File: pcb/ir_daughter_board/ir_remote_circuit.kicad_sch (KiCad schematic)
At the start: 12 parts, among them J2 Conn_01x06, J3 Conn_01x06, SW1 BOOT, SW2 RESET, U3 ESP-WROOM-02

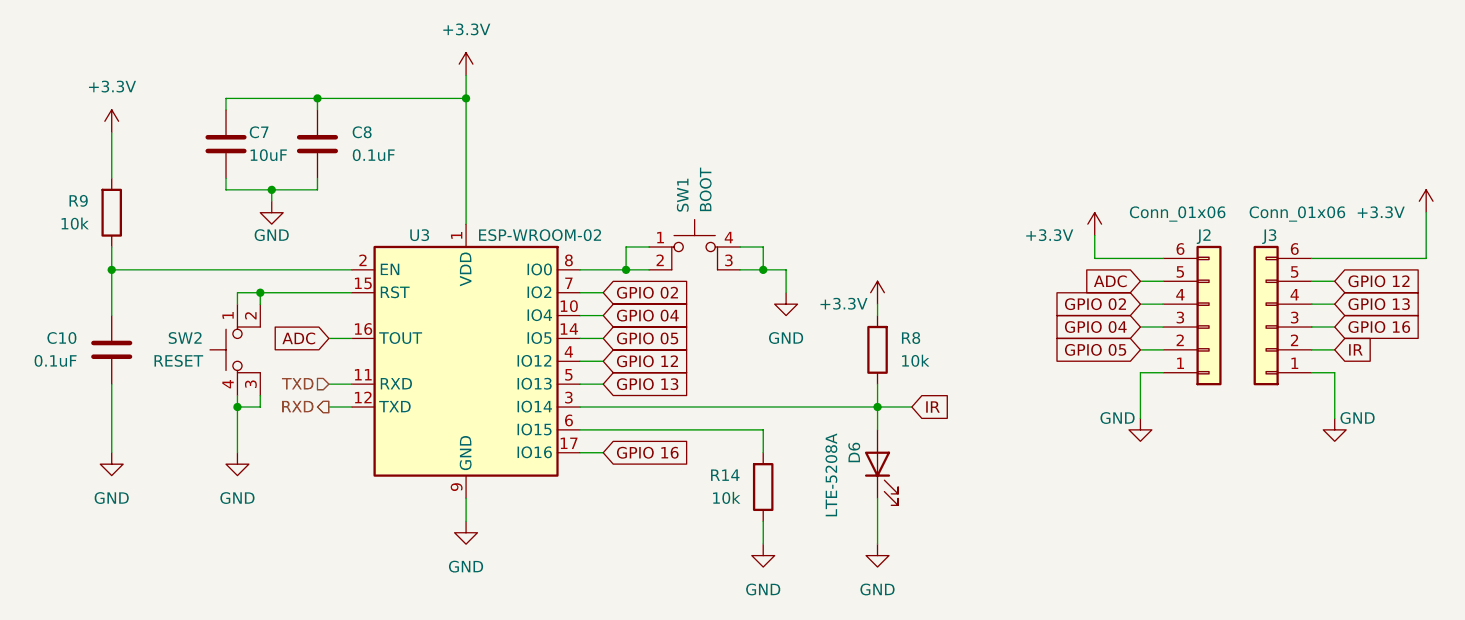
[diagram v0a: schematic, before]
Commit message: updated schematic
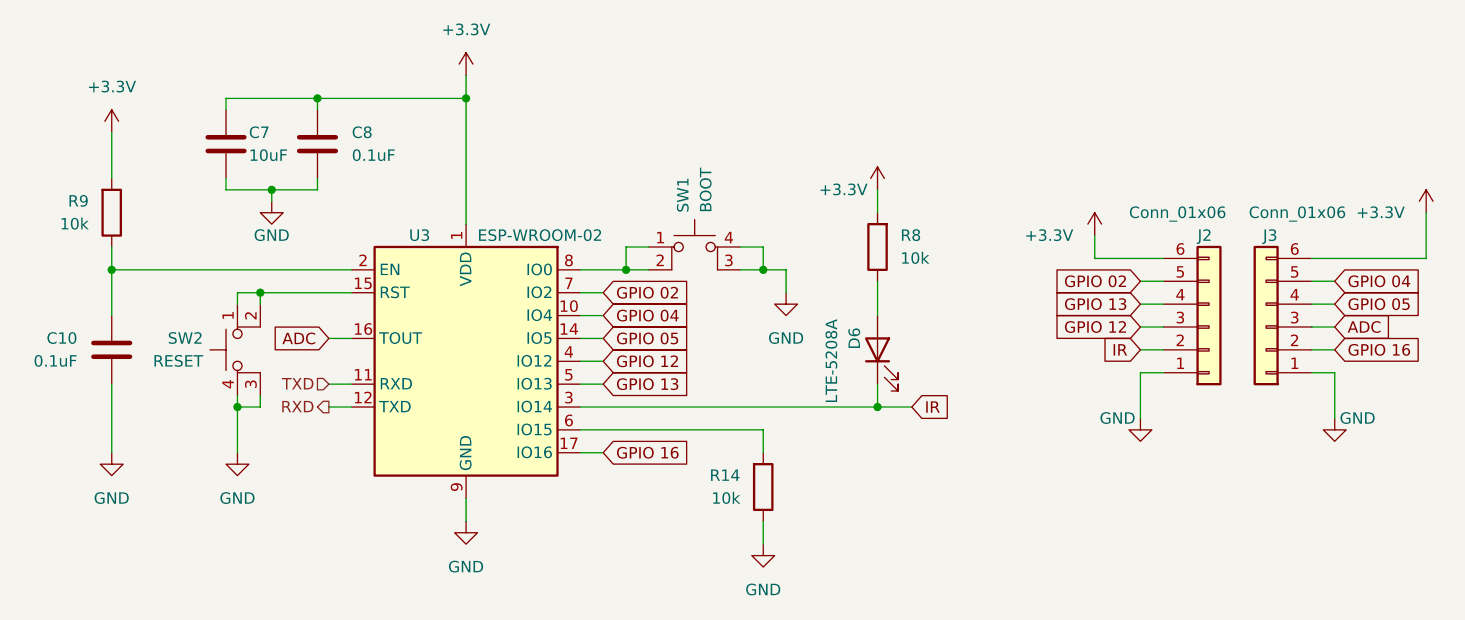
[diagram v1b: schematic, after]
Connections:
- net ADC: now also J3.3 (Pin_3); no longer J2.5 (Pin_5)
- net GND: no longer D6.1 (K)
- net GPIO 02: now also J2.5 (Pin_5); no longer J2.4 (Pin_4)
- net GPIO 04: now also J3.5 (Pin_5); no longer J2.3 (Pin_3)
- net GPIO 05: now also J3.4 (Pin_4); no longer J2.2 (Pin_2)
- net GPIO 12: now also J2.3 (Pin_3); no longer J3.5 (Pin_5)
- net GPIO 13: now also J2.4 (Pin_4); no longer J3.4 (Pin_4)
- net GPIO 16: now also J3.2 (Pin_2); no longer J3.3 (Pin_3)
- net IR: now also D6.1 (K), J2.2 (Pin_2); no longer D6.2 (A), J3.2 (Pin_2), R8.1
- new net: D6.2 (A), R8.1
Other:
- moved on the sheet: D6, R8
